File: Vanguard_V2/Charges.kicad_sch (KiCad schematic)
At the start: 1 part, among them J6 Screw_Terminal_01x04

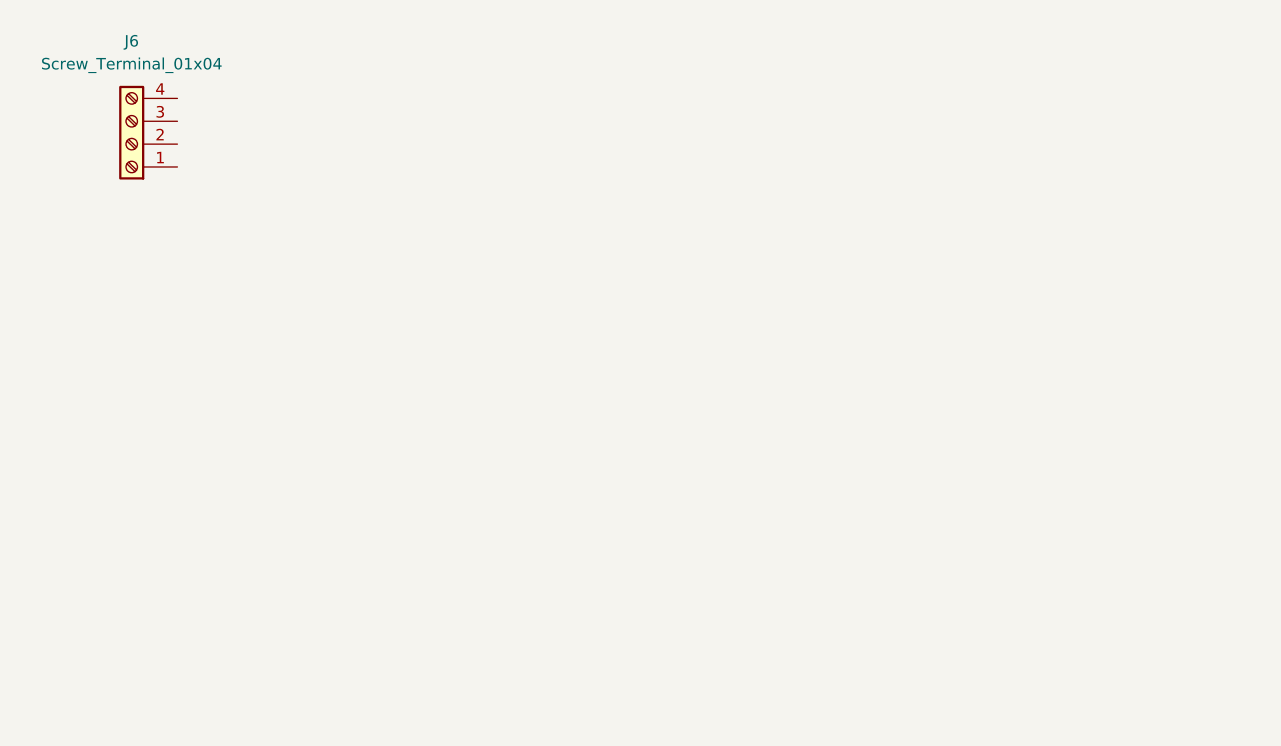
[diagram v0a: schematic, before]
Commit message: started layout for V2.1
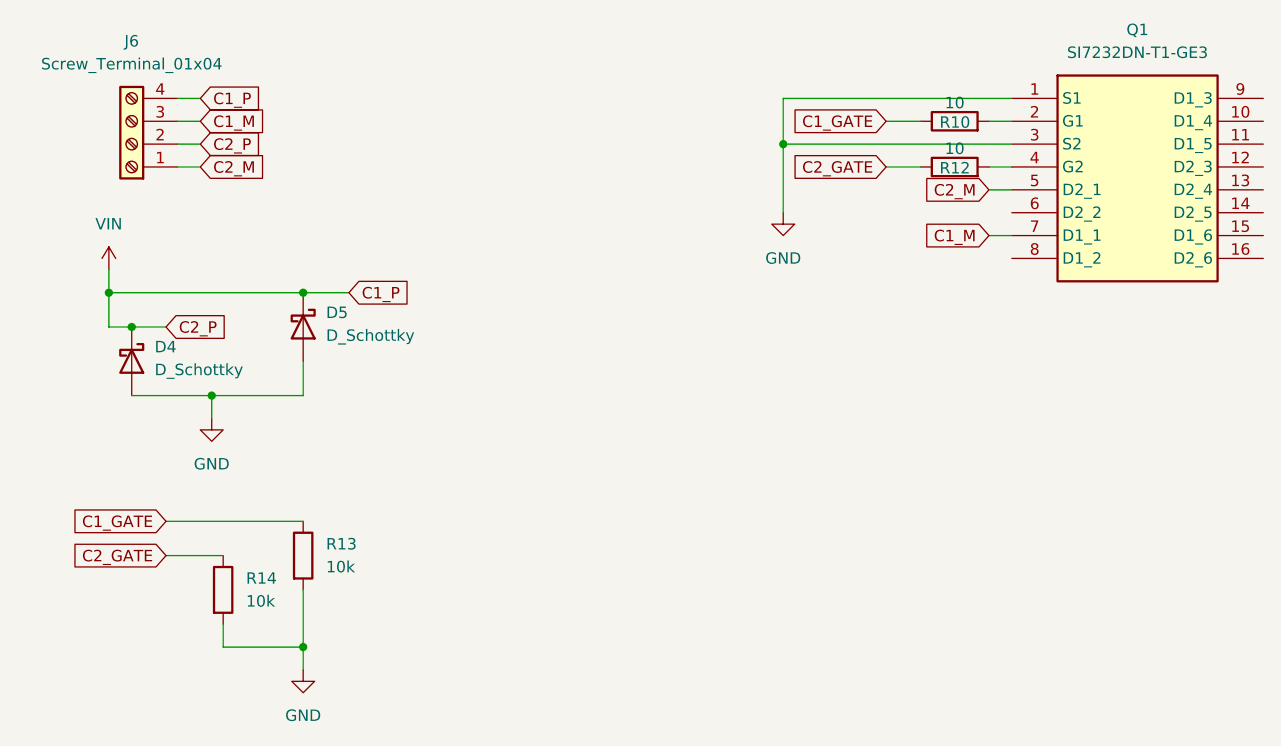
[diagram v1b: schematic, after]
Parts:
- added D4, D5: D_Schottky, Diode_SMD:D_0603_1608Metric, symbol Device:D_Schottky
- added Q1: SI7232DN-T1-GE3, SI7232DNT1GE3, symbol VanguardLib:SI7232DN-T1-GE3
- added R10, R12: 10, Resistor_SMD:R_0402_1005Metric, symbol Device:R
- added R13, R14: 10k, Resistor_SMD:R_0402_1005Metric, symbol Device:R
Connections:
- net C2_M: now reaches J6.1 (Pin_1)
- net C2_M: now also Q1.5 (D2_1)
- net VIN: now reaches J6.2 (Pin_2)
- net VIN: now also J6.4 (Pin_4), D4.1 (K), D5.1 (K)
- net C1_M: now reaches J6.3 (Pin_3)
- net C1_M: now also Q1.7 (D1_1)
- new net: Q1.4 (G2), R12.2
- new net: Q1.2 (G1), R10.2
- new net C1_GATE: R10.1, R13.1
- new net C2_GATE: R12.1, R14.1
- new net GND: D4.2 (A), D5.2 (A), Q1.1 (S1), Q1.3 (S2), R13.2, R14.2
